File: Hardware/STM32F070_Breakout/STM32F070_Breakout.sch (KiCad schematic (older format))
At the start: 29 parts

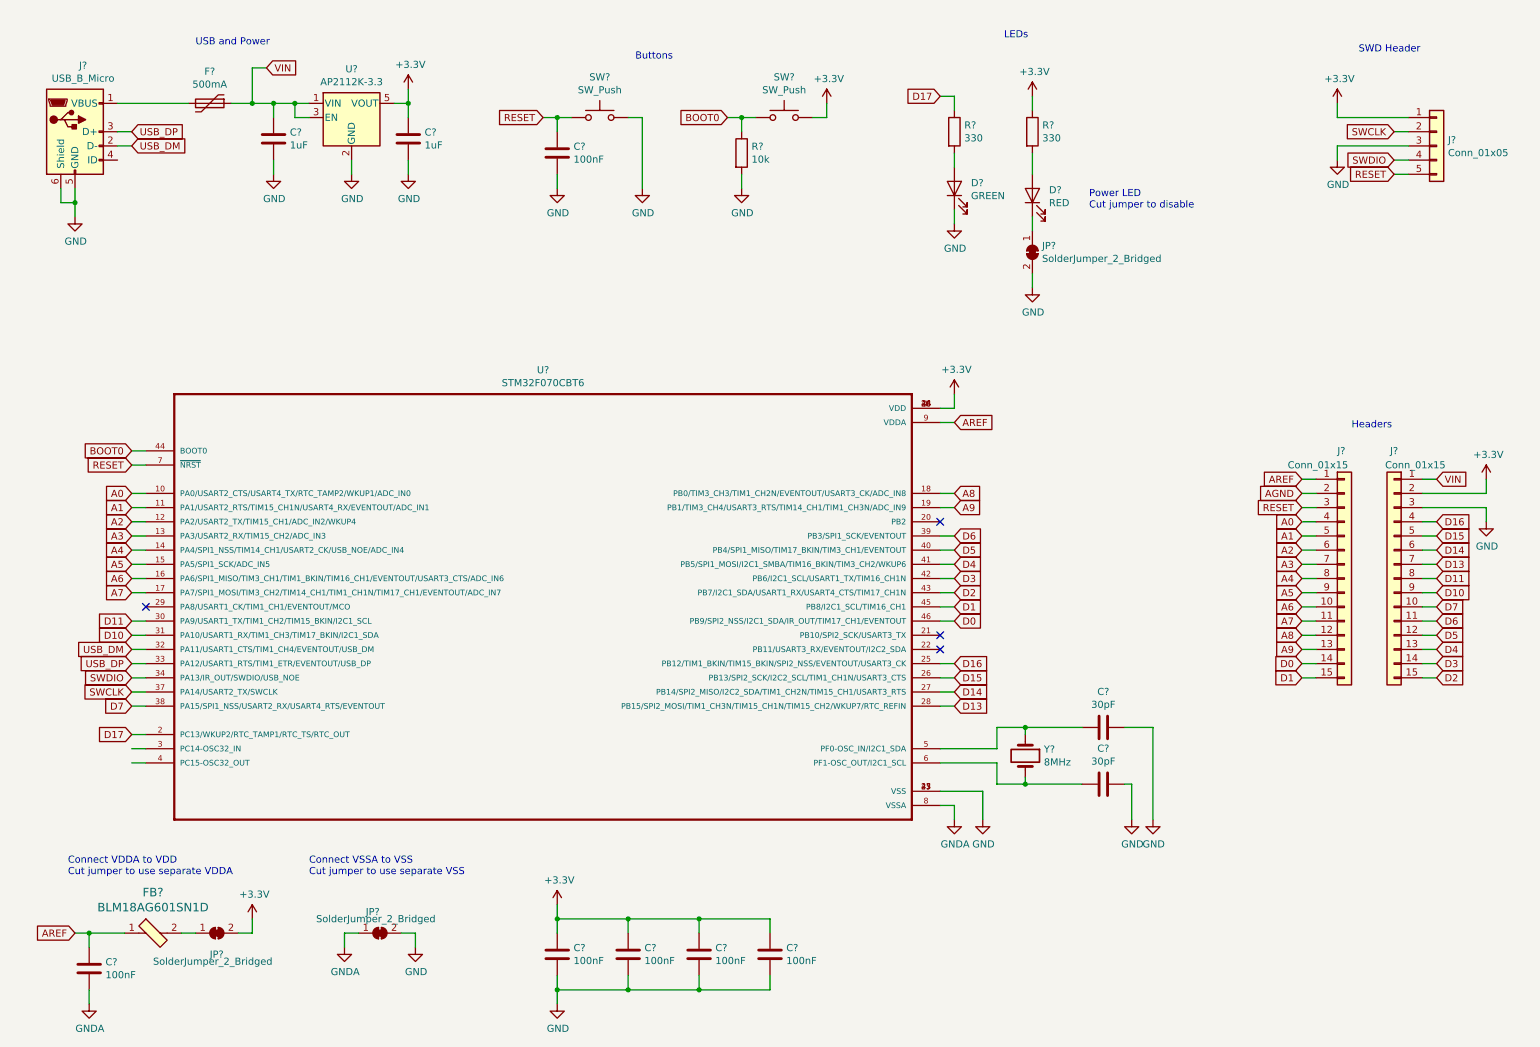
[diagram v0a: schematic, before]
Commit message: Finished schematic
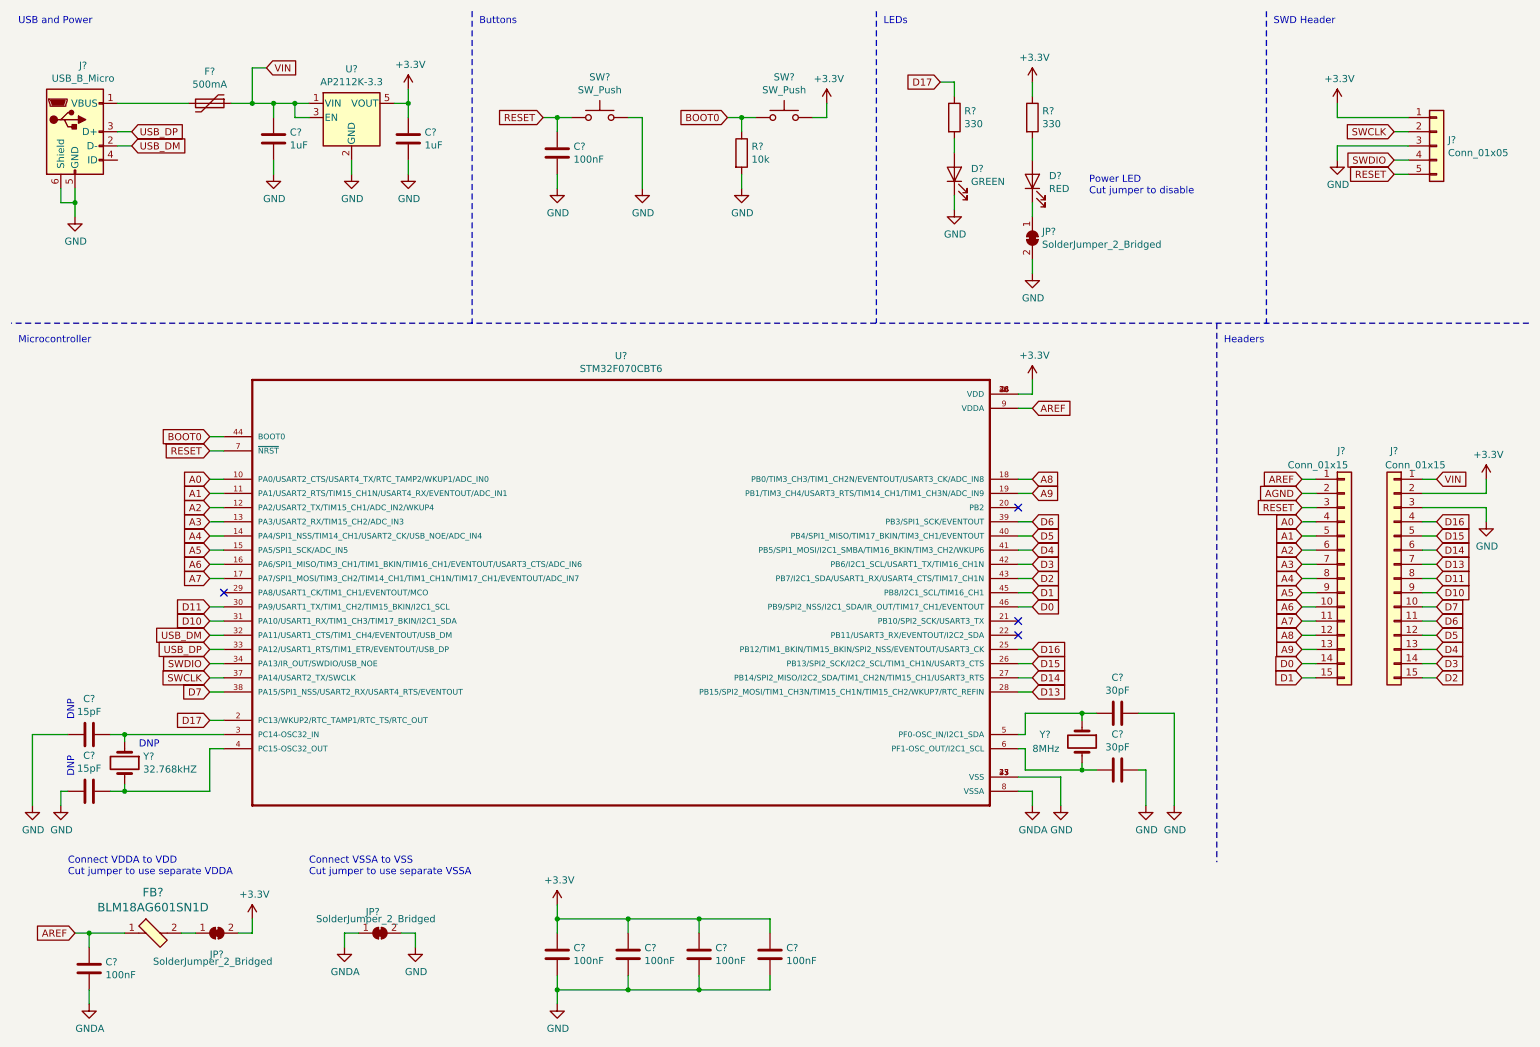
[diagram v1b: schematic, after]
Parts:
- added C? (x2): 15pF, symbol Device:C
- added Y?: 32.768kHZ, symbol Device:Crystal
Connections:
- net GND: now also C?.2, C?.2
- net at U?.3 (PC14-OSC32_IN): now also C?.1, Y?.1
- net at U?.4 (PC15-OSC32_OUT): now also C?.1, Y?.2
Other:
- note added: "Connect VSSA to VSS\nCut jumper to use separate VSSA"
- note added: "DNP"
- note added: "Microcontroller"
- note removed: "Connect VSSA to VSS\nCut jumper to use separate VSS"
- moved on the sheet: C?, D?, JP?, R?, U?, Y?
